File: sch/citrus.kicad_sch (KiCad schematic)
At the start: 1 part, among them J2 ERF8-025-05.0-L-DV-L-K-TR

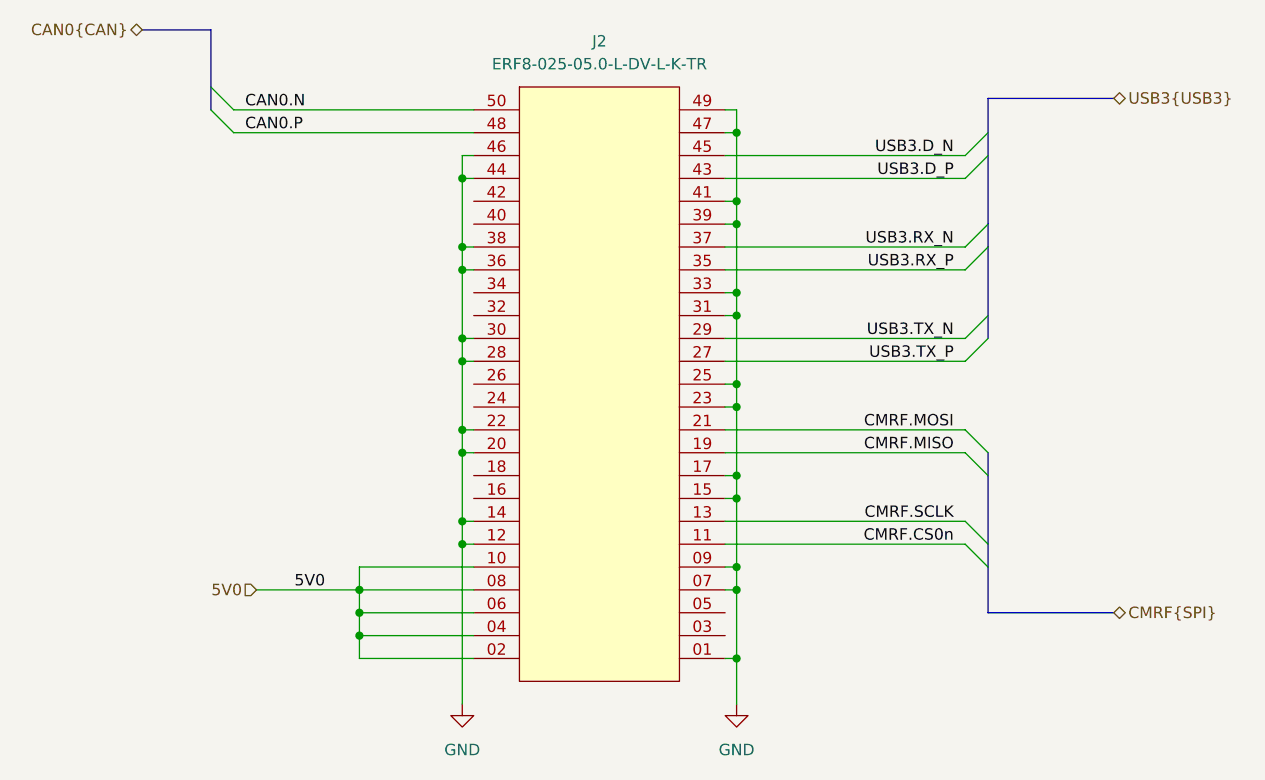
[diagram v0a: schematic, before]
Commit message: added tps and new init layout
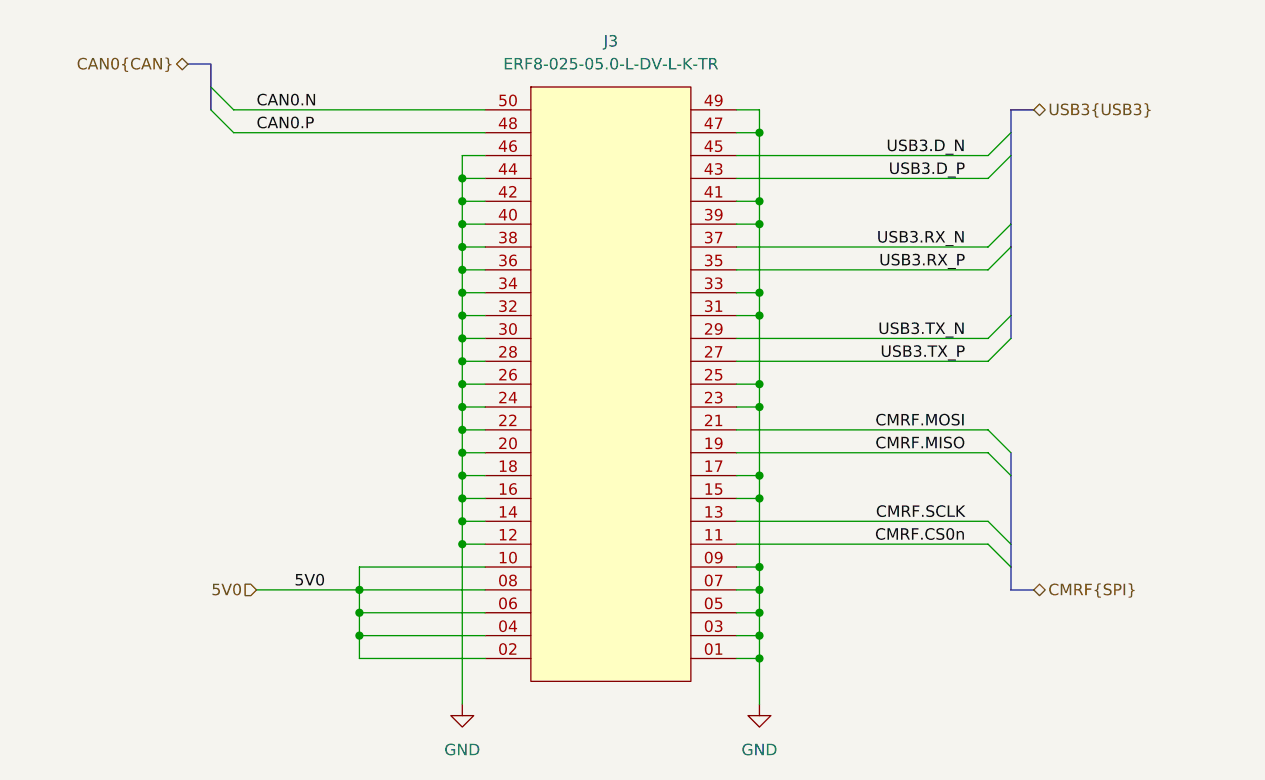
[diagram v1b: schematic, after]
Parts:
- renumbered J2 to J3
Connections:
- net GND: now also J3.03, J3.05, J3.16, J3.18, J3.24, J3.26, J3.32, J3.34, J3.40, J3.42
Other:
- moved on the sheet: J3
